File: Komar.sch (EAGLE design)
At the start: 112 parts, among them CON10 PINHEAD_1X01-2, CON11 PINHEAD_1X01-2, CON12 PINHEAD_1X01-2, CON13 PINHEAD_1X01-2, CON14 PINHEAD_1X01-2, CON15 PINHEAD_1X01-2, CON2 PINHEAD_1X01-2, CON3 CON-4P-TABS-STRAIGHT, CON4 CON-4P-TABS-STRAIGHT, CON5 CON-4P-TABS-STRAIGHT, CON6 CON-4P-TABS-STRAIGHT, CON7 CON-4P-TABS-STRAIGHT, CON8 PINHEAD_1X04-2, CON9 PINHEAD_1X01-2, IC1 TPD3S014DBVR-SOT23-6, IC2 TPD3S014DBVR-SOT23-6, IC3 ATA6561-GBQW-N-HVSON8, IC4 ATA6561-GBQW-N-HVSON8, IC5 MCP9700AT-E/TTVAO-SOT23, IC6 11LC040T-E/TT, J1 105133-0011, Q1 FDMS86368-F085, Q10 FDMS86368-F085, Q11 FDMS86368-F085, Q12 FDMS86368-F085, Q2 FDMS86368-F085, Q3 FDMS86368-F085, Q4 FDMS86368-F085, Q5 FDMS86368-F085, Q6 FDMS86368-F085, Q7 FDMS86368-F085, Q8 FDMS86368-F085, Q9 FDMS86368-F085

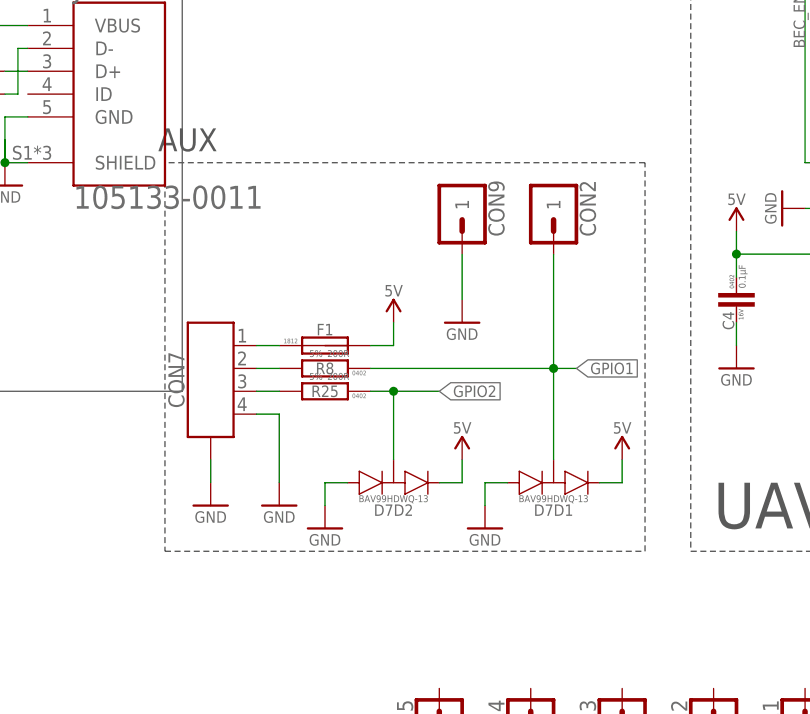
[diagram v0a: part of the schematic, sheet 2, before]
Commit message: minor changes to fixes #26
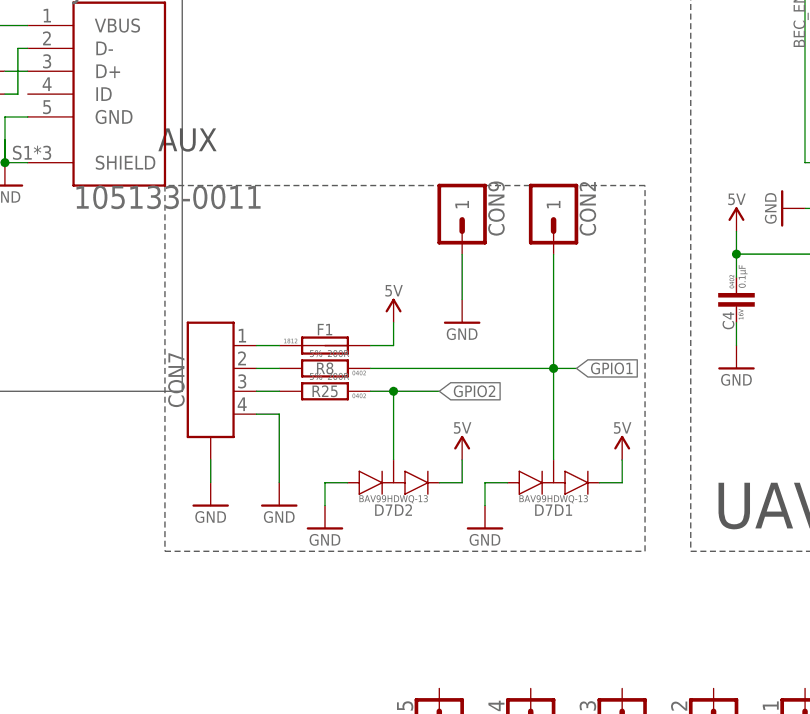
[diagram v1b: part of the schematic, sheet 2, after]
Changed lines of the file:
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@@
 <setting verticaltext="up"/>
 </settings>
-<grid distance="1" unitdist="mm" unit="mm" style="lines" multiple="1" display="no" altdistance="0.1" altunitdist="mm" altunit="mm"/>
+<grid distance="0.1" unitdist="inch" unit="inch" style="lines" multiple="1" display="no" altdistance="0.01" altunitdist="inch" altunit="inch"/>
 <layers>
 <layer number="1" name="Top" color="4" fill="1" visible="no" active="no"/>
@@
 <text x="142.24" y="160.02" size="2.54" layer="97">Place close to power mosfets</text>
 <text x="182.88" y="76.2" size="2.54" layer="97" font="vector" ratio="15" align="center">AUX</text>
-<wire x1="180.34" y1="73.66" x2="180.34" y2="30.48" width="0.1524" layer="97" style="shortdash"/>
+<wire x1="180.34" y1="71.12" x2="180.34" y2="30.48" width="0.1524" layer="97" style="shortdash"/>
 <wire x1="180.34" y1="30.48" x2="233.68" y2="30.48" width="0.1524" layer="97" style="shortdash"/>
-<wire x1="233.68" y1="30.48" x2="233.68" y2="73.66" width="0.1524" layer="97" style="shortdash"/>
-<wire x1="233.68" y1="73.66" x2="180.34" y2="73.66" width="0.1524" layer="97" style="shortdash"/>
+<wire x1="233.68" y1="30.48" x2="233.68" y2="71.12" width="0.1524" layer="97" style="shortdash"/>
+<wire x1="233.68" y1="71.12" x2="180.34" y2="71.12" width="0.1524" layer="97" style="shortdash"/>
 <text x="5.08" y="269.24" size="2.54" layer="97" font="vector" ratio="15" align="center-left">Power should be connected with multi-strand 12AWG wire in silicone insulation</text>
 <text x="68.58" y="276.86" size="2.54" layer="97" font="vector" ratio="15" align="center">PCB hole diameters for wires are based on the chart from PCBLibraries.com
